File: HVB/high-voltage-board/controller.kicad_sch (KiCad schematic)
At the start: 25 parts, among them J10 FTSH-107-01-F-DV-k, J12 Conn_01x02, Q3 DMN3404L, U1 MAX33054EASA+T, U4 LD1117S33TR_SOT223, U5 STM32F413CGUx, Y1 CSTME8M00

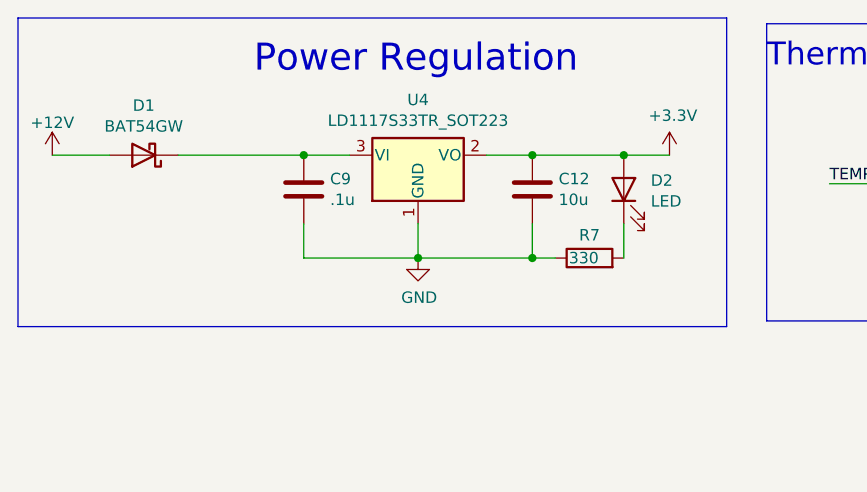
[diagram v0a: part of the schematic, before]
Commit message: touching up layout and making gerbers
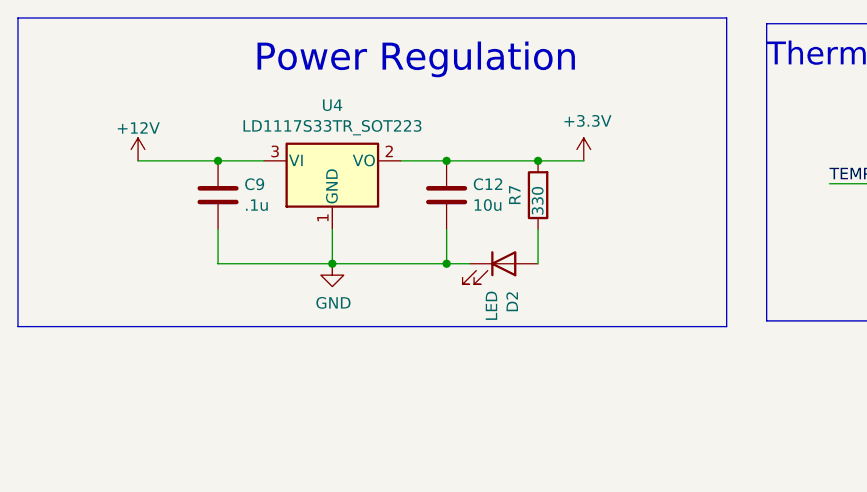
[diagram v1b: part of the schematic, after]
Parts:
- removed D1: BAT54GW, Diode_SMD:D_SOD-123, symbol Device:D_Schottky
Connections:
- net +12V: now also C9.1, U4.3 (VI)
- net +3V3: now also R7.2; no longer D2.2 (A)
- net GND: now also D2.1 (K); no longer R7.1
- new net: D2.2 (A), R7.1
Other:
- moved on the sheet: C12, C9, D2, R7, U4
